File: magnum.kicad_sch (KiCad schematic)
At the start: 0 parts

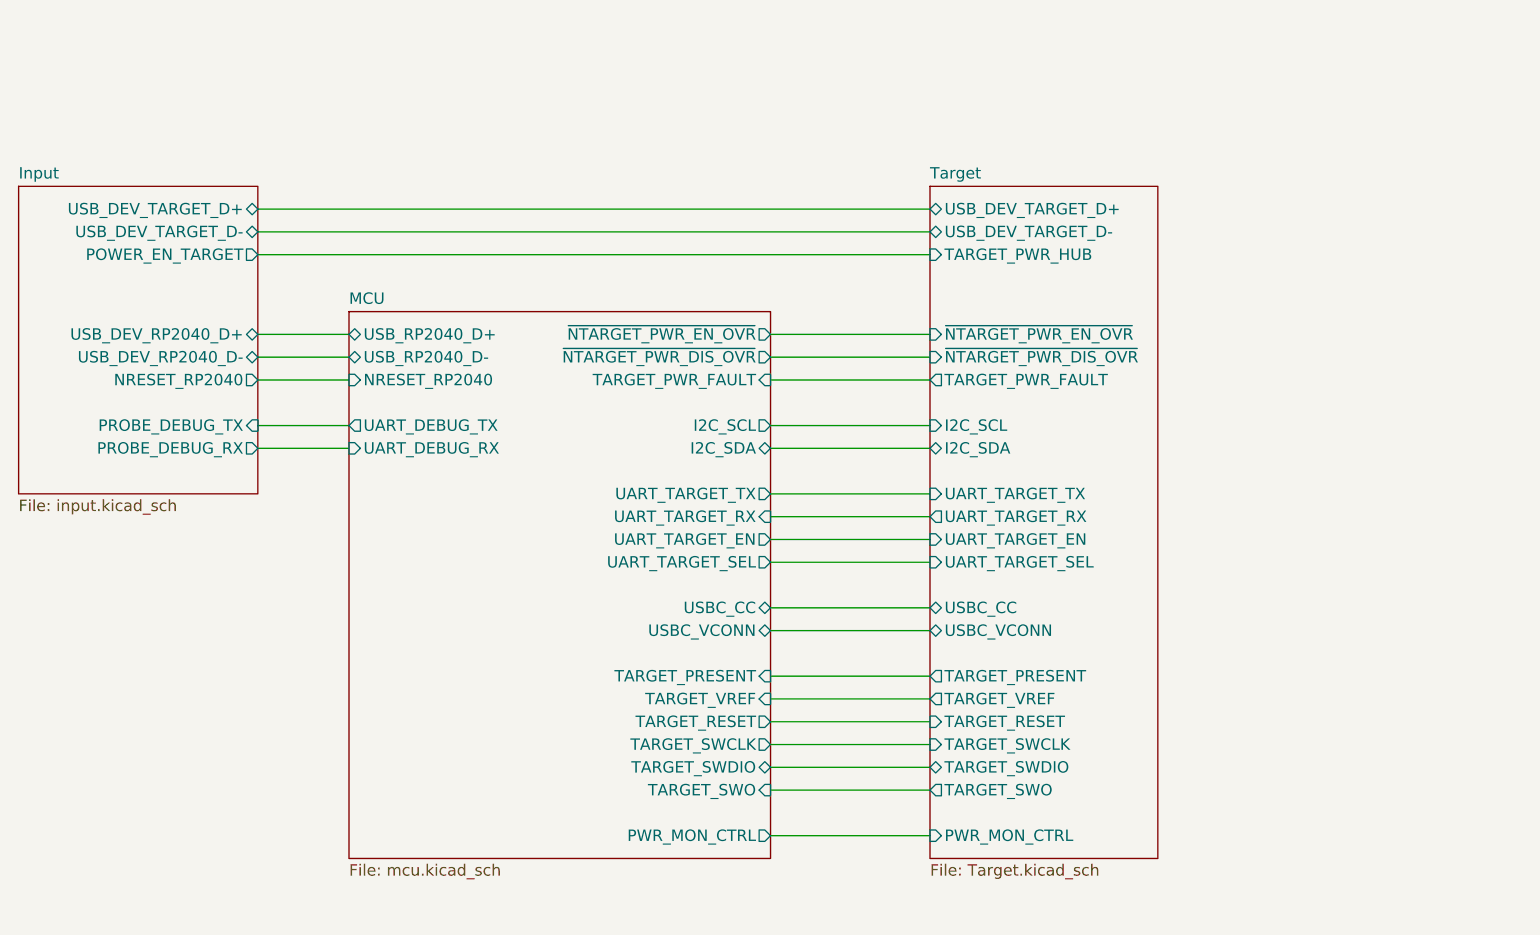
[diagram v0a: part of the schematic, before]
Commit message: Changes and updates for revision 1 release
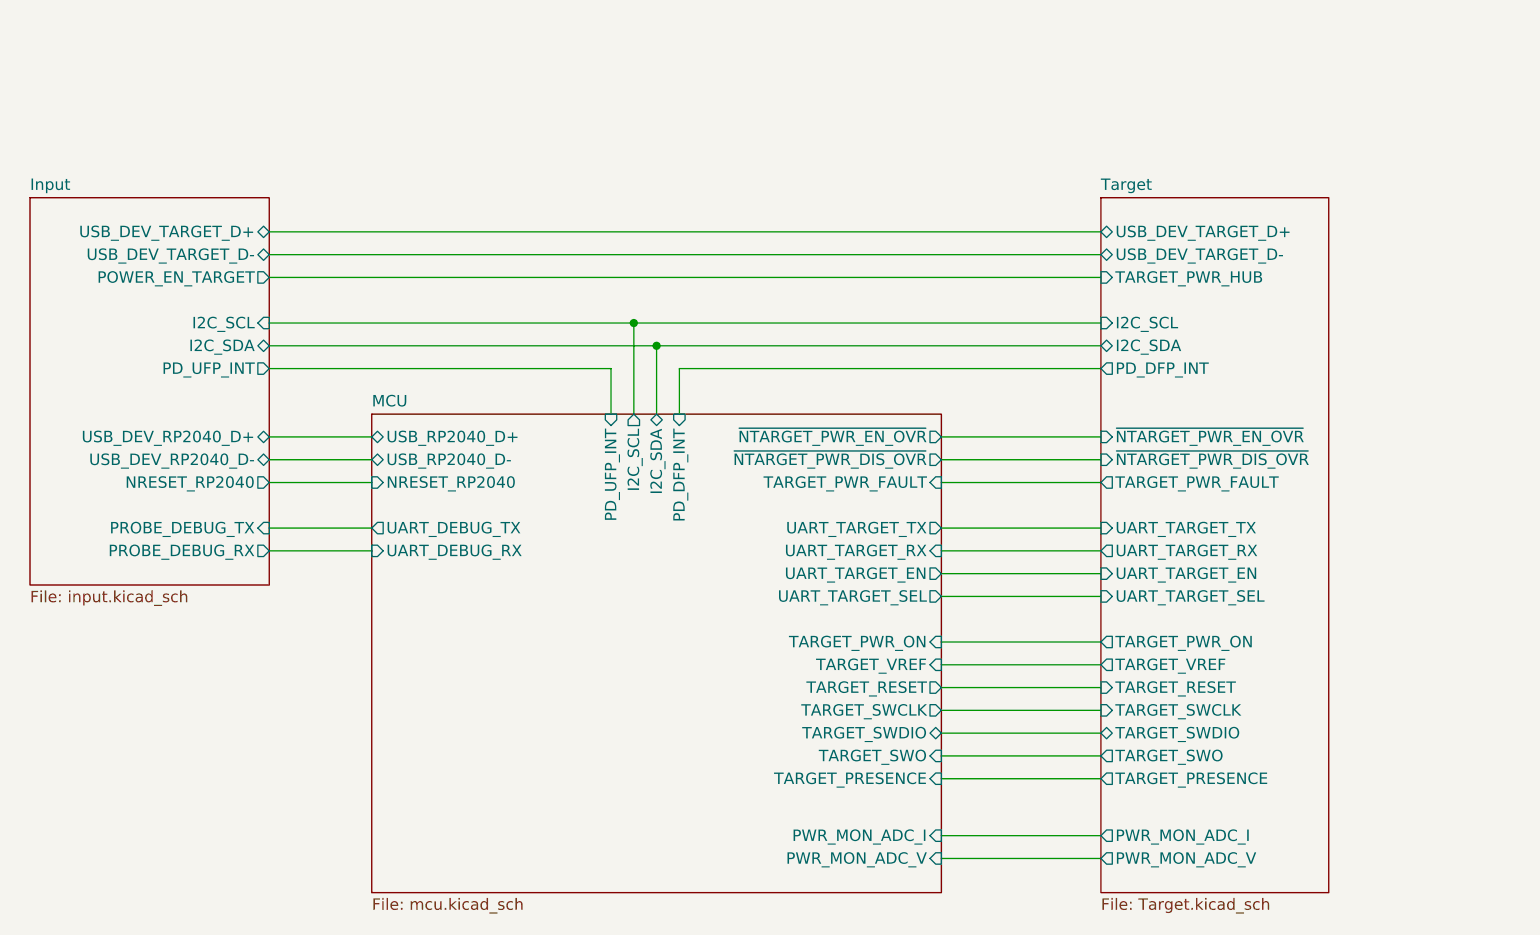
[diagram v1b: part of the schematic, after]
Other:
- sheet Input ports: added I2C_SCL, I2C_SDA, PD_UFP_INT; removed none
- sheet MCU ports: added PD_DFP_INT, PD_UFP_INT, PWR_MON_ADC_I, PWR_MON_ADC_V, TARGET_PRESENCE, TARGET_PWR_ON; removed PWR_MON_CTRL, TARGET_PRESENT, USBC_CC, USBC_VCONN
- sheet Target ports: added PD_DFP_INT, PWR_MON_ADC_I, PWR_MON_ADC_V, TARGET_PRESENCE, TARGET_PWR_ON; removed PWR_MON_CTRL, TARGET_PRESENT, USBC_CC, USBC_VCONN
- company: (none) -> Redhill Embedded
- title: (none) -> Magnum
